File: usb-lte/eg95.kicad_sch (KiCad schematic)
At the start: 25 parts, among them J2 Conn_Coaxial, J3 Conn_Coaxial, J4 Conn_Coaxial, U2 EG95

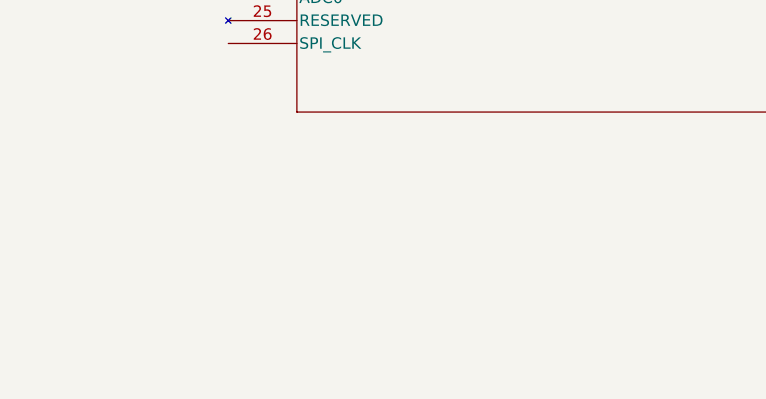
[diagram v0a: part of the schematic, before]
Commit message: Add various test points
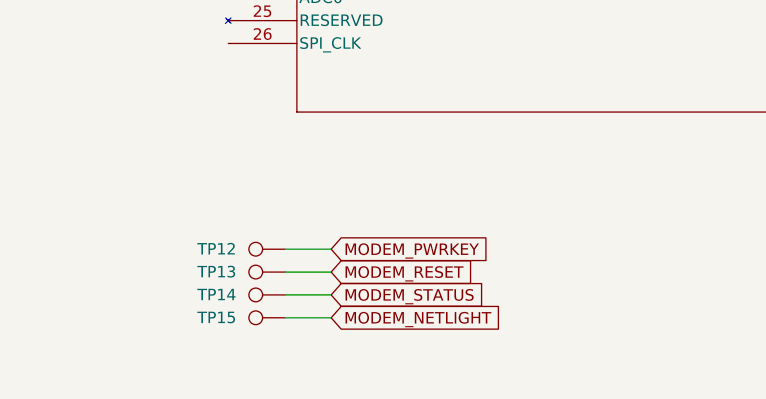
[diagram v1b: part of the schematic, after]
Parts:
- added TP12, TP13, TP14, TP15: TestPoint, footprints:TestPoint_Pad_1mm, symbol Connector:TestPoint
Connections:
- net MODEM_NETLIGHT: now also TP15.1
- net MODEM_PWRKEY: now also TP12.1
- net MODEM_RESET: now also TP13.1
- net MODEM_STATUS: now also TP14.1

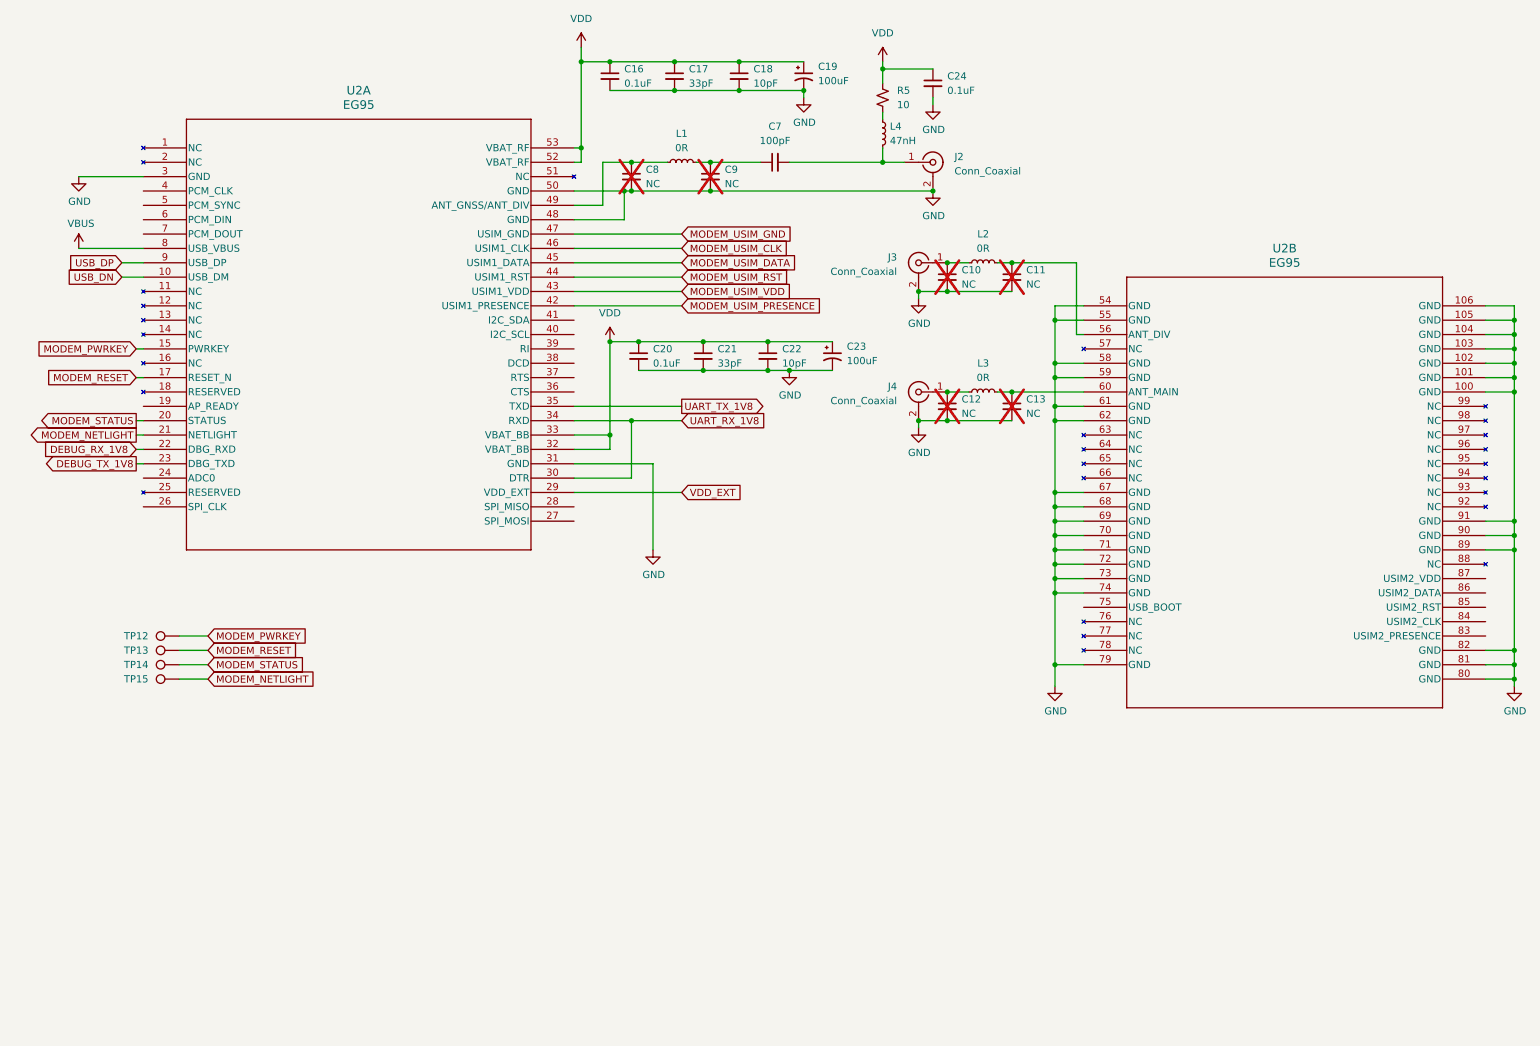
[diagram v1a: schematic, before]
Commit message: Update 3d models
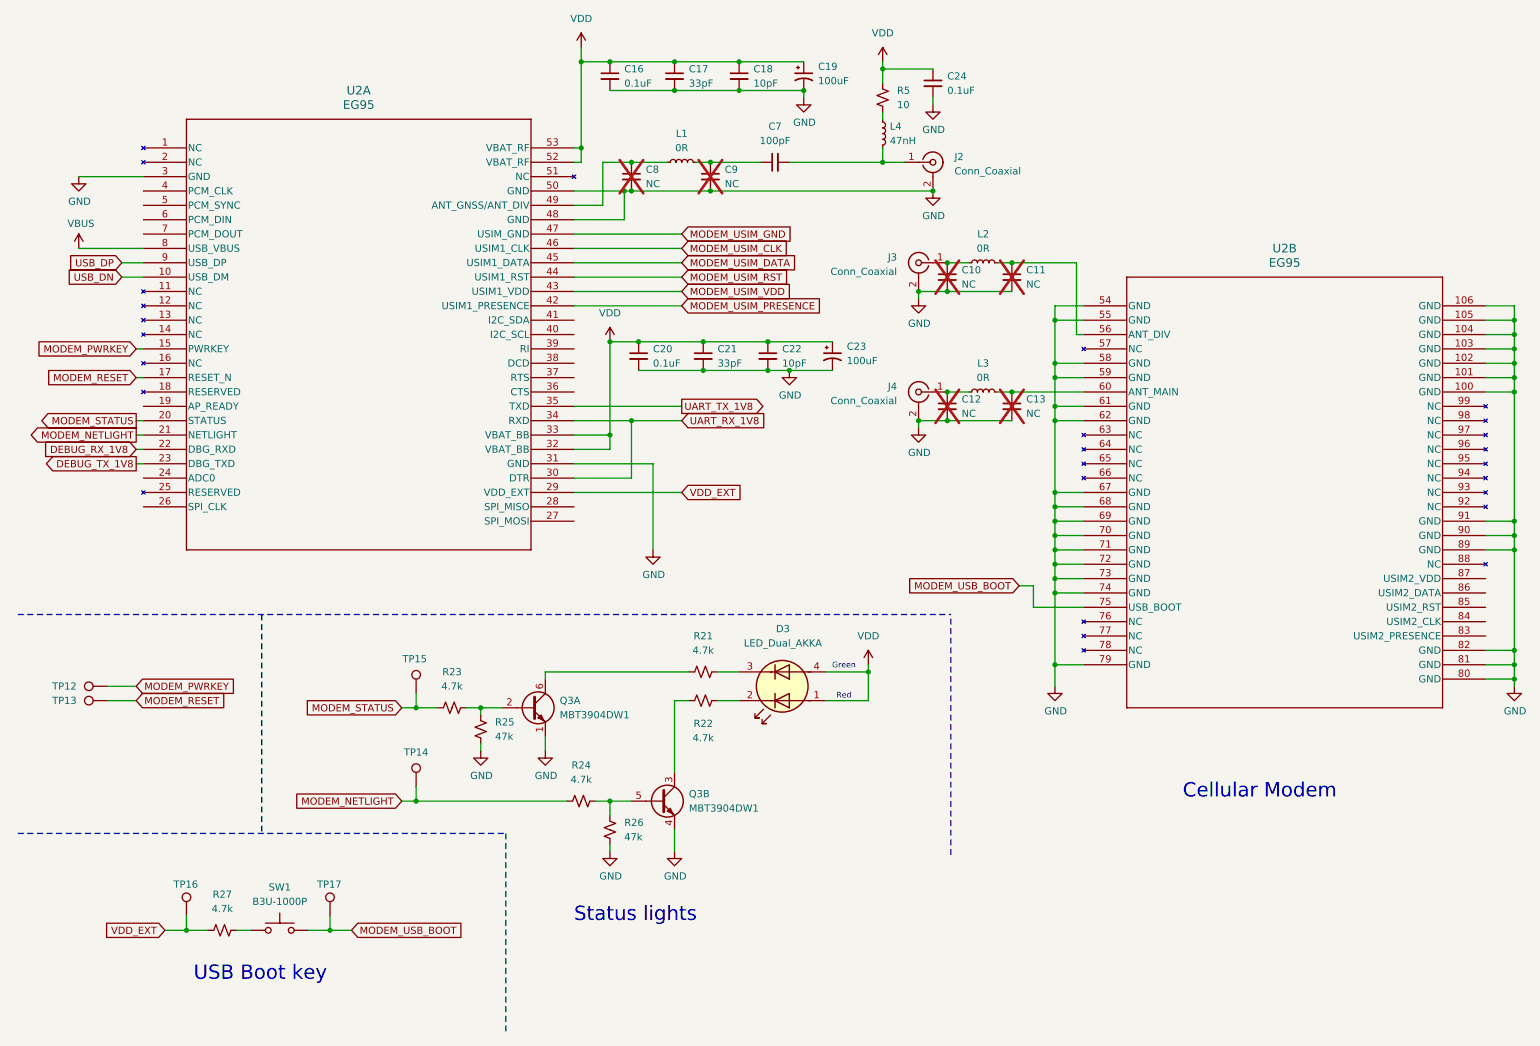
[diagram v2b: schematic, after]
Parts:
- added D3: LED_Dual_AKKA, footprints:LED_Dual_0805_4pin, symbol Device:LED_Dual_AKKA
- added Q3: MBT3904DW1, Package_TO_SOT_SMD:SOT-363_SC-70-6, symbol Transistor_BJT:MBT3904DW1
- added R21, R22, R23, R24, R27: 4.7k, Resistor_SMD:R_0402_1005Metric, symbol Device:R_Small_US
- added R25, R26: 47k, Resistor_SMD:R_0402_1005Metric, symbol Device:R_Small_US
- added SW1: B3U-1000P, Button_Switch_SMD:SW_SPST_B3U-1000P, symbol Switch:SW_Push
- added TP16, TP17: TestPoint, footprints:TestPoint_Pad_1mm, symbol Connector:TestPoint
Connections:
- net GND: now also Q3.1 (E1), Q3.4 (E2), R25.1, R26.1
- net MODEM_NETLIGHT: now also TP14.1, R24.2; no longer TP15.1
- net MODEM_STATUS: now also TP15.1, R23.2; no longer TP14.1
- net VDD: now also D3.1 (A1), D3.4 (A2)
- net VDD_EXT: now also R27.2, TP16.1
- net MODEM_USB_BOOT: now reaches U2.75 (USB_BOOT)
- net MODEM_USB_BOOT: now also SW1.2, TP17.1
- new net: Q3.2 (B1), R23.1, R25.2
- new net: Q3.5 (B2), R24.1, R26.2
- new net: Q3.6 (C1), R21.2
- new net: D3.2 (K1), R22.1
- new net: Q3.3 (C2), R22.2
- new net: R27.1, SW1.1
- new net: D3.3 (K2), R21.1
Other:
- note added: "Cellular Modem"
- note added: "Green"
- note added: "Red"
- note added: "Status lights"
- note added: "USB Boot key"
- title: Framework LTE Expansion Card -> Framework Cellular Expansion Card
- moved on the sheet: TP12, TP13, TP14, TP15
